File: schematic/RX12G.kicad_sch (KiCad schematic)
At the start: 11 parts, among them J1 ICSP, U1 PIC32MK1024GPK064-I/PT, X1 24 MHz

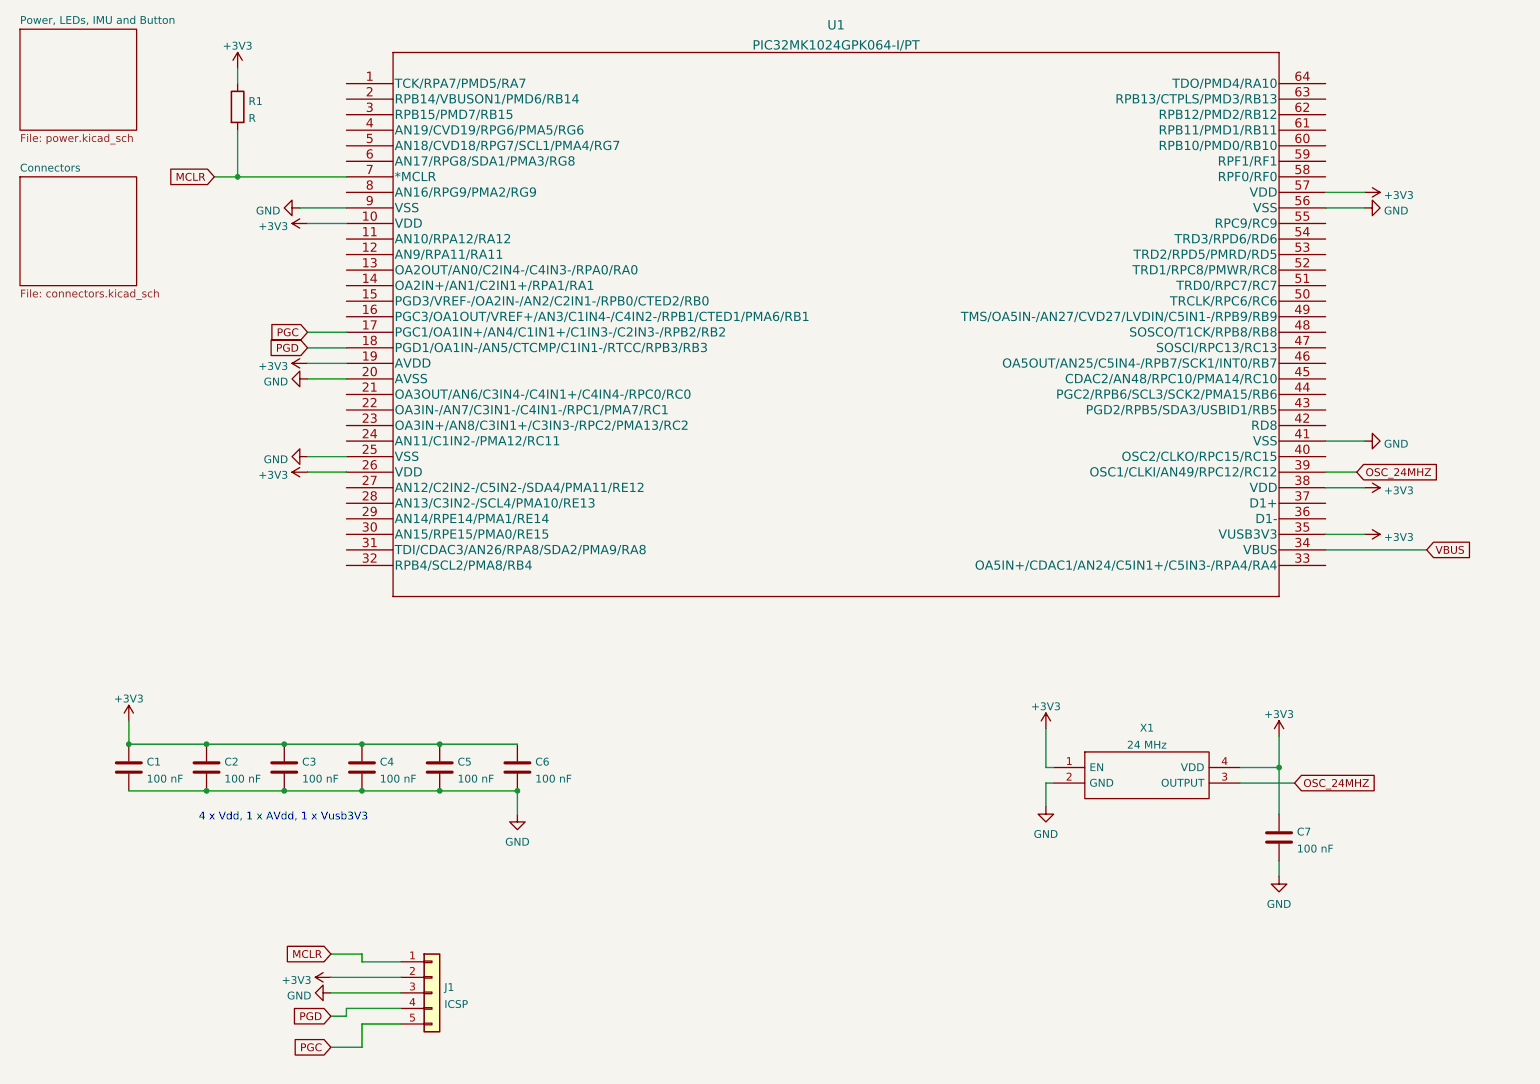
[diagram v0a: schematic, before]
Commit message: Complete schematic
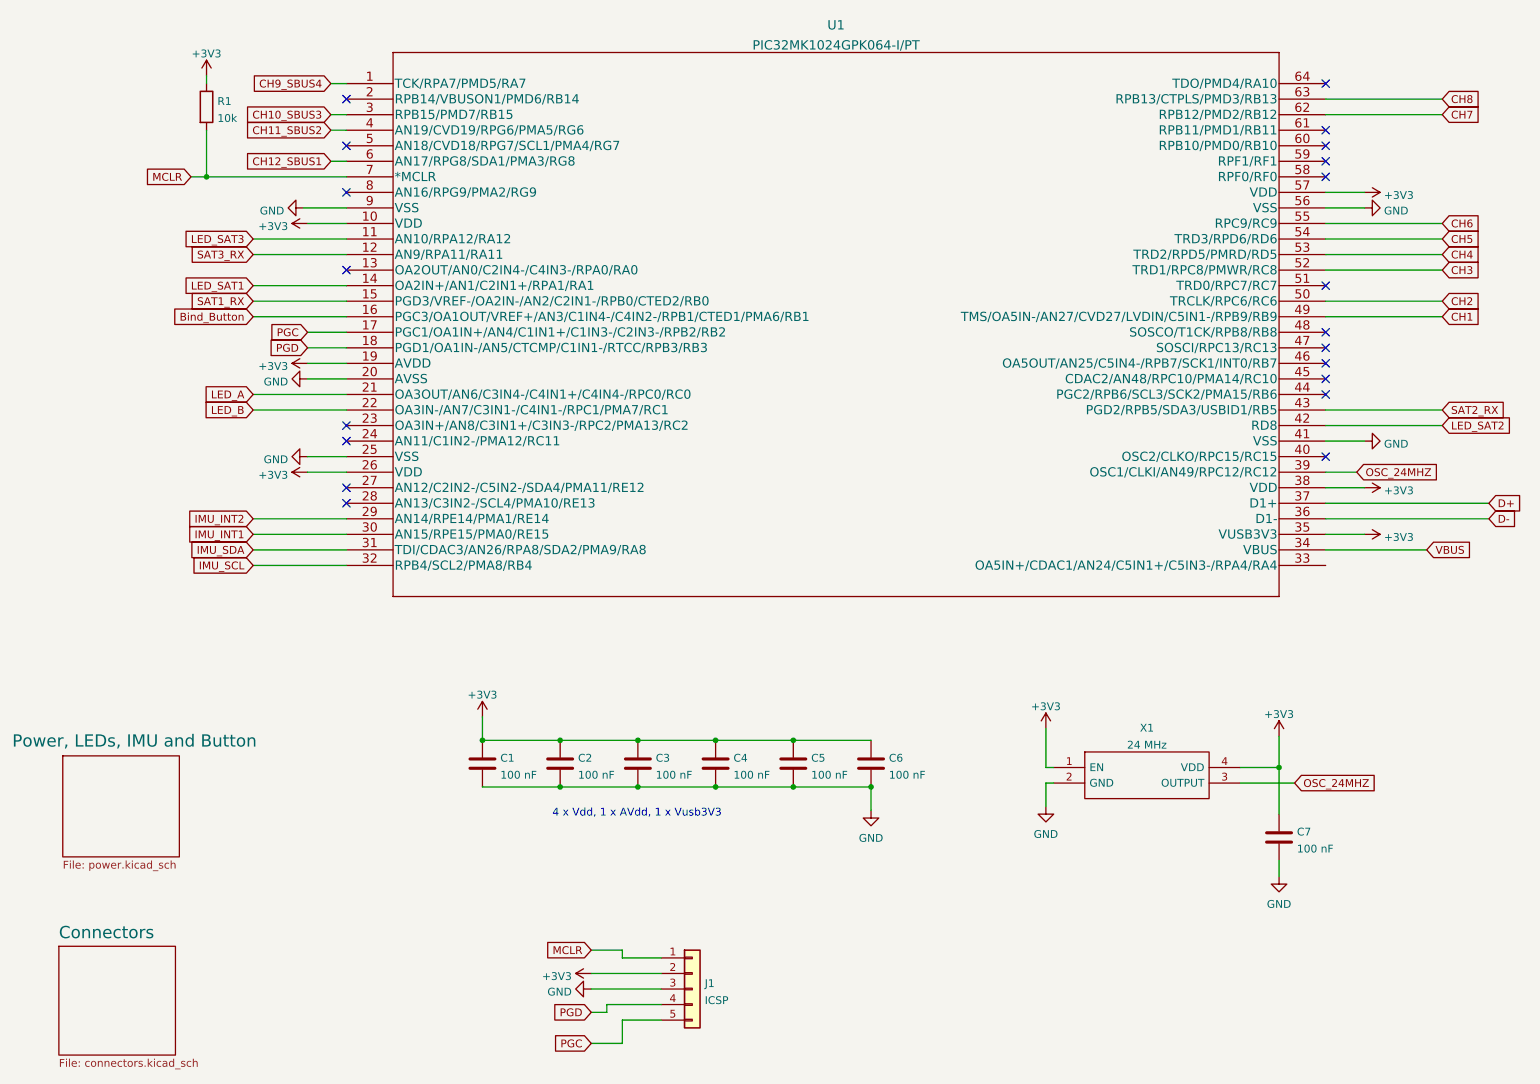
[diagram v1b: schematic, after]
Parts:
- C1, C2, C3, C4, C5, C6, C7: footprint (none) -> Capacitor_SMD:C_0402_1005Metric
- J1: footprint (none) -> Connector_PinHeader_2.54mm:PinHeader_1x05_P2.54mm_Vertical
- R1: value R -> 10k; footprint (none) -> Resistor_SMD:R_0603_1608Metric
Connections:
- net CH9_SBUS4: now reaches U1.1 (TCK/RPA7/PMD5/RA7)
- net LED_SAT3: now reaches U1.11 (AN10/RPA12/RA12)
- net SAT3_RX: now reaches U1.12 (AN9/RPA11/RA11)
- net LED_SAT1: now reaches U1.14 (OA2IN+/AN1/C2IN1+/RPA1/RA1)
- net SAT1_RX: now reaches U1.15 (PGD3/VREF-/OA2IN-/AN2/C2IN1-/RPB0/CTED2/RB0)
- net Bind_Button: now reaches U1.16 (PGC3/OA1OUT/VREF+/AN3/C1IN4-/C4IN2-/RPB1/CTED1/PMA6/RB1)
- net LED_A: now reaches U1.21 (OA3OUT/AN6/C3IN4-/C4IN1+/C4IN4-/RPC0/RC0)
- net LED_B: now reaches U1.22 (OA3IN-/AN7/C3IN1-/C4IN1-/RPC1/PMA7/RC1)
- net IMU_INT2: now reaches U1.29 (AN14/RPE14/PMA1/RE14)
- net CH10_SBUS3: now reaches U1.3 (RPB15/PMD7/RB15)
- net IMU_INT1: now reaches U1.30 (AN15/RPE15/PMA0/RE15)
- net IMU_SDA: now reaches U1.31 (TDI/CDAC3/AN26/RPA8/SDA2/PMA9/RA8)
- net IMU_SCL: now reaches U1.32 (RPB4/SCL2/PMA8/RB4)
- net D-: now reaches U1.36 (D1-)
- net D+: now reaches U1.37 (D1+)
- net CH11_SBUS2: now reaches U1.4 (AN19/CVD19/RPG6/PMA5/RG6)
- net LED_SAT2: now reaches U1.42 (RD8)
- net SAT2_RX: now reaches U1.43 (PGD2/RPB5/SDA3/USBID1/RB5)
- net CH1: now reaches U1.49 (TMS/OA5IN-/AN27/CVD27/LVDIN/C5IN1-/RPB9/RB9)
- net CH2: now reaches U1.50 (TRCLK/RPC6/RC6)
- net CH3: now reaches U1.52 (TRD1/RPC8/PMWR/RC8)
- net CH4: now reaches U1.53 (TRD2/RPD5/PMRD/RD5)
- net CH5: now reaches U1.54 (TRD3/RPD6/RD6)
- net CH6: now reaches U1.55 (RPC9/RC9)
- net CH12_SBUS1: now reaches U1.6 (AN17/RPG8/SDA1/PMA3/RG8)
- net CH7: now reaches U1.62 (RPB12/PMD2/RB12)
- net CH8: now reaches U1.63 (RPB13/CTPLS/PMD3/RB13)
- no-connect marks 0 -> 20
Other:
- moved on the sheet: C1, C2, C3, C4, C5, C6, J1, R1
